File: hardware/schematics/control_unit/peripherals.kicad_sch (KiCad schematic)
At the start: 14 parts, among them Q17 IRFZ44N, Q18 2N7000, U13 PC817, U14 MAX487E

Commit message: !feat
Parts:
- D5, D6: footprint Diode_THT:D_DO-41_SOD81_P10.16mm_Horizontal -> Diode_THT:D_DO-41_SOD81_P7.62mm_Horizontal
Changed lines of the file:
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@@
 			)
 		)
-		(property "Footprint" "Diode_THT:D_DO-41_SOD81_P10.16mm_Horizontal"
+		(property "Footprint" "Diode_THT:D_DO-41_SOD81_P7.62mm_Horizontal"
 			(at 161.925 114.3 0)
 			(effects
@@
 			)
 		)
-		(property "Footprint" "Diode_THT:D_DO-41_SOD81_P10.16mm_Horizontal"
+		(property "Footprint" "Diode_THT:D_DO-41_SOD81_P7.62mm_Horizontal"
 			(at 113.665 114.3 0)
 			(effects

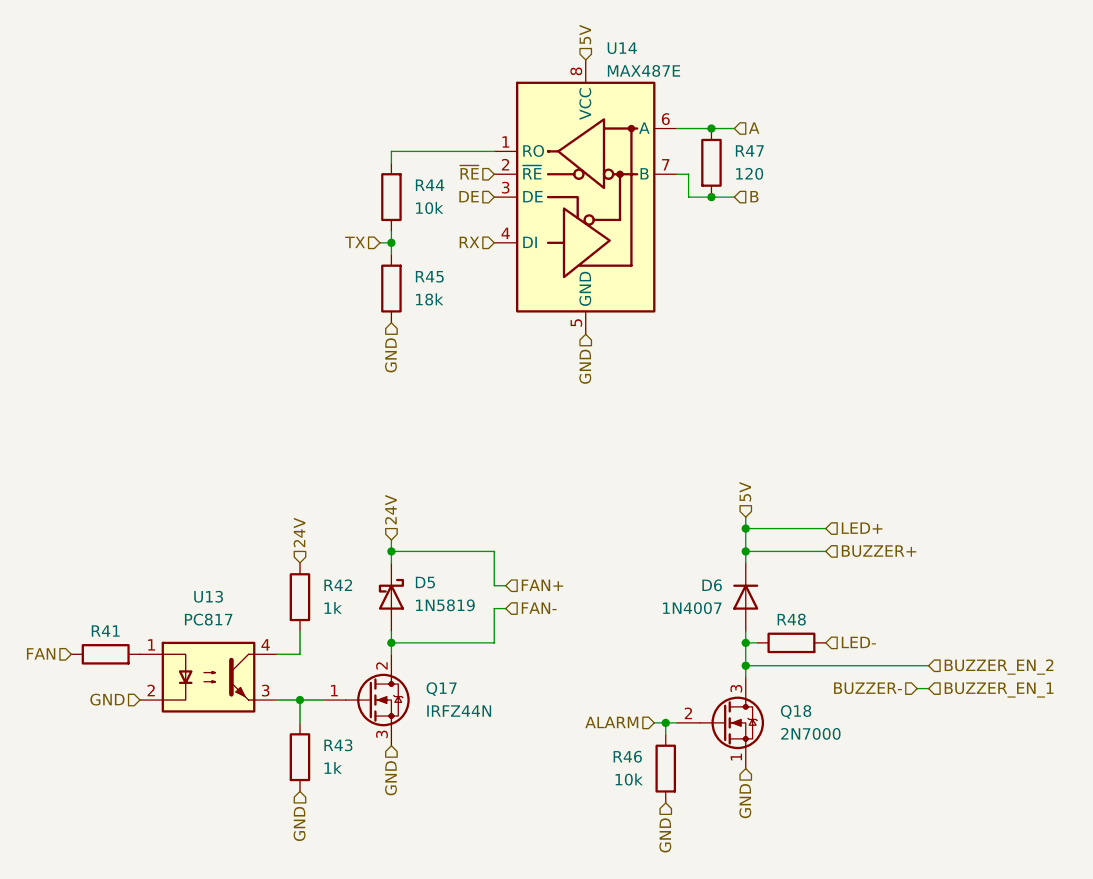
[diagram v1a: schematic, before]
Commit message: !feat
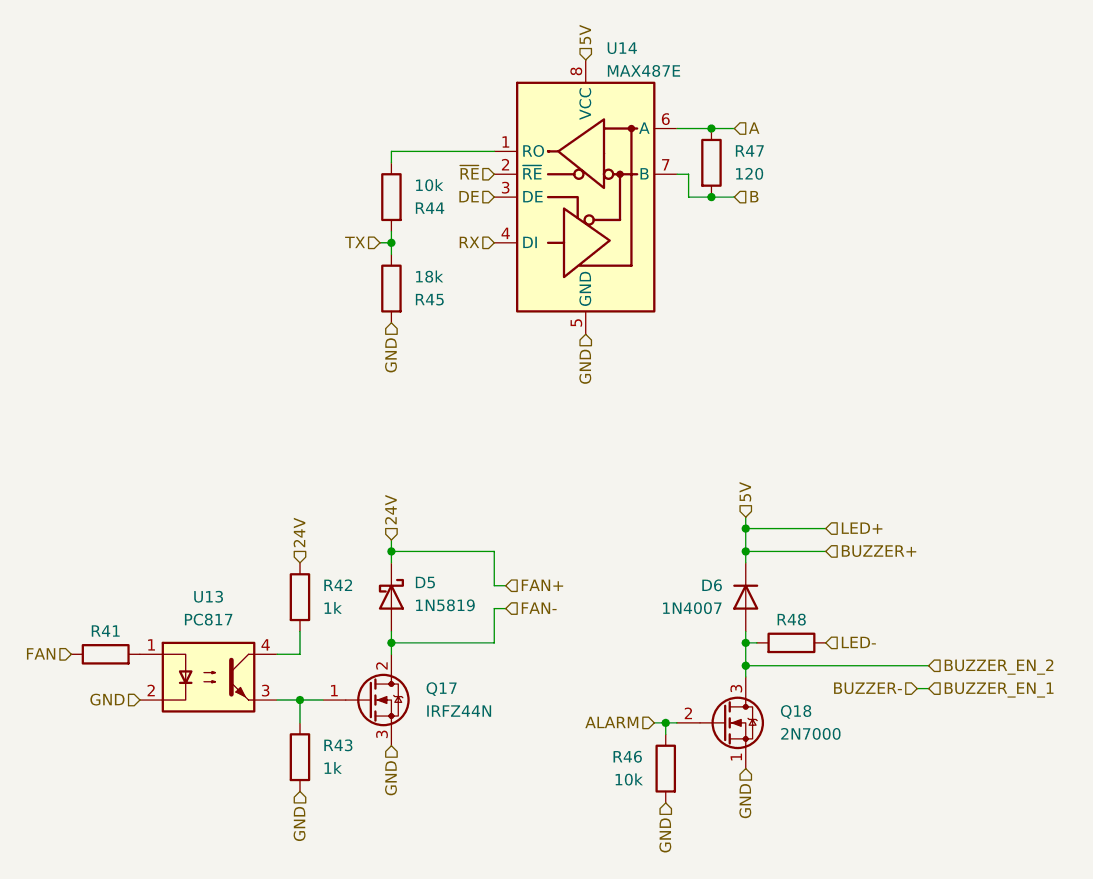
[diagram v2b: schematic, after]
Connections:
- net BUZZER_EN_2: now also R48.2; no longer R48.1
- net GND: now also R45.2; no longer R45.1
- net LED-: now also R48.1; no longer R48.2
- net TX: now also R44.2, R45.1; no longer R44.1, R45.2
- net at U14.1 (RO): now also R44.1; no longer R44.2
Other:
- moved on the sheet: R44, R45, R48
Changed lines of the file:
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@@
 	(symbol
 		(lib_id "Device:R")
-		(at 162.56 119.38 90)
+		(at 162.56 119.38 270)
+		(mirror x)
 		(unit 1)
 		(exclude_from_sim no)
@@
 	(symbol
 		(lib_id "Device:R")
-		(at 118.11 69.85 180)
+		(at 118.11 69.85 0)
+		(mirror y)
 		(unit 1)
 		(exclude_from_sim no)
@@
 		(dnp no)
 		(property "Reference" "R44"
-			(at 120.65 68.5799 0)
+			(at 120.65 71.1201 0)
 			(effects
 				(font
@@
 		)
 		(property "Value" "10k"
-			(at 120.65 71.1199 0)
+			(at 120.65 68.5801 0)
 			(effects
 				(font
@@
 	(symbol
 		(lib_id "Device:R")
-		(at 118.11 80.01 180)
+		(at 118.11 80.01 0)
+		(mirror y)
 		(unit 1)
 		(exclude_from_sim no)
@@
 		(dnp no)
 		(property "Reference" "R45"
-			(at 120.65 78.7399 0)
+			(at 120.65 81.2801 0)
 			(effects
 				(font
@@
 		)
 		(property "Value" "18k"
-			(at 120.65 81.2799 0)
-			(effects
-				(font
+			(at 120.65 78.7401 0)
+			(effects
+				(font
